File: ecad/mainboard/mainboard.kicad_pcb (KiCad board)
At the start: 4 copper layers, 340 x 220 mm, 122 parts, among them J1 TYPE-C-31-M-12, J2 SWD, J3 UART, SW1 BOOTSEL, SW2 RUN, SW3 Key_Switch_with_LED, SW4 Key_Switch_with_LED, U1 NCP1117-3.3_SOT223, U10 DRV5056A3xQDBZxR, U11 DRV5056A3xQDBZxR, U12 DRV5056A3xQDBZxR, U13 DRV5056A3xQDBZxR, U14 DRV5056A3xQDBZxR, U15 DRV5056A3xQDBZxR, U16 DRV5056A3xQDBZxR, U17 DRV5056A3xQDBZxR, U18 DRV5056A3xQDBZxR, U19 DRV5056A3xQDBZxR, U2 USBLC6-2SC6, U20 DRV5056A3xQDBZxR, U21 DRV5056A3xQDBZxR, U22 CD4051BM96, U23 CD4051BM96, U3 W25Q128JVS, U4 74AHCT1G125, U5 RP2040, U6 DRV5056A3xQDBZxR, U7 DRV5056A3xQDBZxR, U8 DRV5056A3xQDBZxR, U9 DRV5056A3xQDBZxR, Y1 ABM8-272-T3

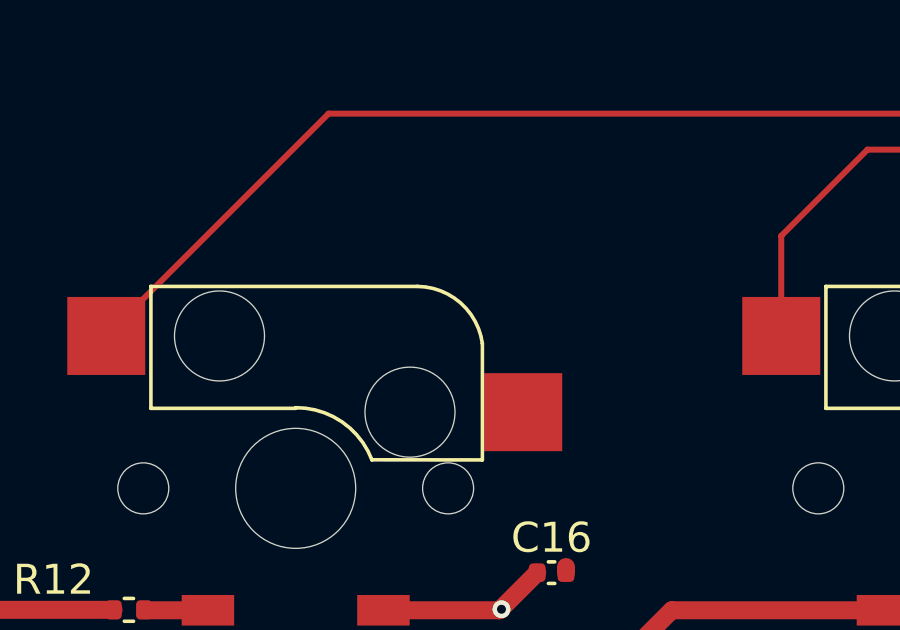
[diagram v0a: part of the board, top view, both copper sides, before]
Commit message: .
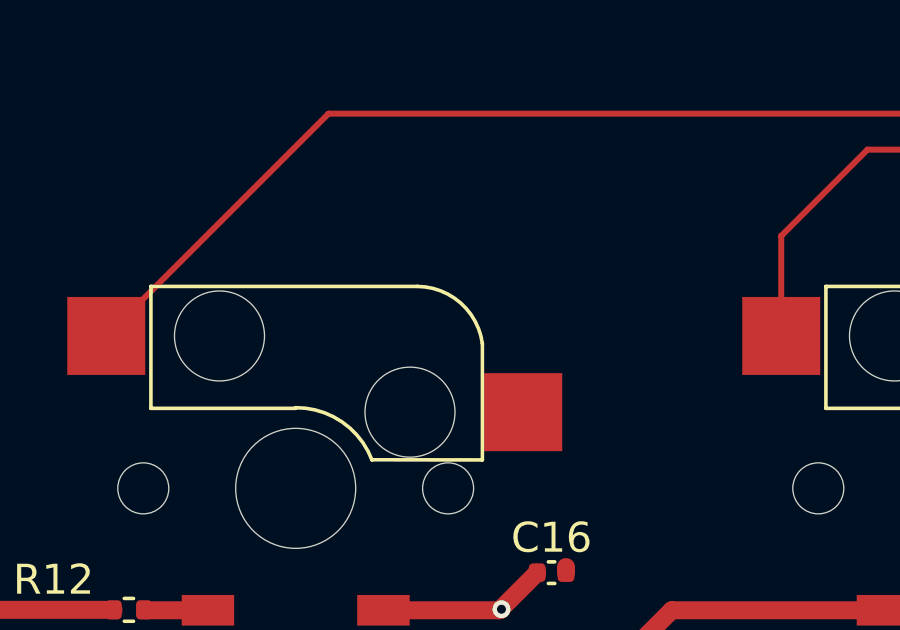
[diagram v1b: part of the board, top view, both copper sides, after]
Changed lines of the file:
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@@
 			(disableapertmacros no)
 			(usegerberextensions no)
-			(usegerberattributes yes)
+			(usegerberattributes no)
 			(usegerberadvancedattributes yes)
 			(creategerberjobfile yes)
@@
 			(outputformat 1)
 			(mirror no)
-			(drillshape 1)
+			(drillshape 0)
 			(scaleselection 1)
-			(outputdirectory "")
+			(outputdirectory "gerber/")
 		)
 	)
@@
 		(fp_arc
 			(start 5.436 16.231)
-			(mid 4.002296 15.679932)
+			(mid 4.002293 15.679933)
 			(end 3.277 14.326)
 			(stroke
